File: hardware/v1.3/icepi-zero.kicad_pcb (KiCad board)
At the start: 4 copper layers, 65 x 30 mm, 162 parts, among them J1 Conn_02x20_Counter_Clockwise, J2 GPDI_C_1.3, J3 USB_C_Receptacle_USB2.0_14P, J4 USB_C_Receptacle_USB2.0_14P, J5 USB_C_Receptacle_USB2.0_14P, J6 Micro_SD_Card_Det2, SW1 SW_Push, SW2 SW_Push, U1 ECP5-CABGA256, U10 W9825G6KH, U11 W25Q128JVS, U2 TLV62569DBV, U3 TLV62569DBV, U4 TLV62569DBV, U5 PCA9306DC1, U6 FT231XQ, U7 TPD2EUSB30A, U8 TPD2EUSB30A, U9 TPD2EUSB30A, Y1 SG-8018CG 50.000000MHz

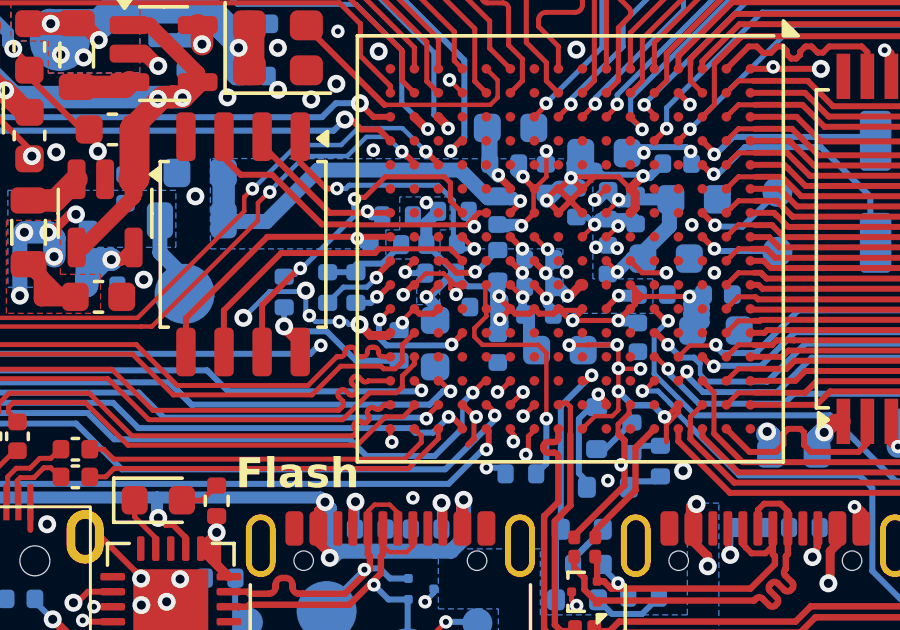
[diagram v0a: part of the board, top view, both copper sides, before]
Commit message: DVI multires
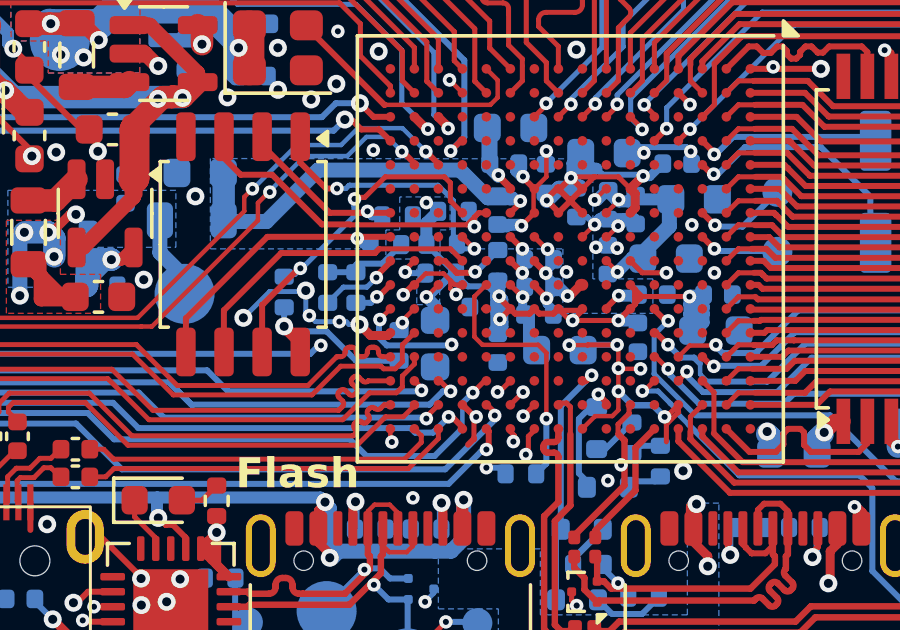
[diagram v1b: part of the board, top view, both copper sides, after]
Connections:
- U1 pad M11: /USB/JTAG_TDO -> unconnected-(U1E-PR47A/+/HS/RSQ44-PadM11)
- U1 pad N12: /USB/JTAG_TMS -> unconnected-(U1E-PR44D/-/RSQ44-PadN12)
- U1 pad P11: /USB/JTAG_TDI -> unconnected-(U1E-PR47C/+/RSQ44/LRC_GPLL0T_IN-PadP11)
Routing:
- net /USB/JTAG_TDI: track 32.6 -> 31.7 mm
- net /USB/JTAG_TMS: track 34.5 -> 34.0 mm
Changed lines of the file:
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@@
 	(net 259 "/GPIO27")
 	(net 260 "unconnected-(U1J-PB18A{slash}WRITEN-PadM9)")
+	(net 261 "unconnected-(U1E-PR44D{slash}-{slash}RSQ44-PadN12)")
+	(net 262 "unconnected-(U1E-PR47C{slash}+{slash}RSQ44{slash}LRC_GPLL0T_IN-PadP11)")
+	(net 263 "unconnected-(U1E-PR47A{slash}+{slash}HS{slash}RSQ44-PadM11)")
 	(footprint "MountingHole:MountingHole_2.7mm_M2.5"
 		(layer "F.Cu")
@@
 			(property pad_prop_bga)
 			(layers "F.Cu" "F.Mask" "F.Paste")
-			(net 5 "/USB/JTAG_TDO")
+			(net 263 "unconnected-(U1E-PR47A{slash}+{slash}HS{slash}RSQ44-PadM11)")
 			(pinfunction "PR47A/+/HS/RSQ44")
 			(pintype "bidirectional")
@@
 			(property pad_prop_bga)
 			(layers "F.Cu" "F.Mask" "F.Paste")
-			(net 8 "/USB/JTAG_TMS")
+			(net 261 "unconnected-(U1E-PR44D{slash}-{slash}RSQ44-PadN12)")
 			(pinfunction "PR44D/-/RSQ44")
 			(pintype "bidirectional")
@@
 			(property pad_prop_bga)
 			(layers "F.Cu" "F.Mask" "F.Paste")
-			(net 4 "/USB/JTAG_TDI")
+			(net 262 "unconnected-(U1E-PR47C{slash}+{slash}RSQ44{slash}LRC_GPLL0T_IN-PadP11)")
 			(pinfunction "PR47C/+/RSQ44/LRC_GPLL0T_IN")
 			(pintype "bidirectional")
@@
 		(net 4)
 	)
-	(segment
-		(start 144.96 106.91)
-		(end 144.8 106.75)
-		(width 0.2)
-		(layer "F.Cu")
-		(net 4)
-	)
-	(segment
-		(start 145.44 106.91)
-		(end 144.96 106.91)
-		(width 0.2)
-		(layer "F.Cu")
-		(net 4)
-	)
-	(segment
-		(start 145.6 106.75)
-		(end 145.44 106.91)
-		(width 0.2)
-		(layer "F.Cu")
-		(net 4)
-	)
 	(via
 		(at 144.399998 107.209961)
@@
 	)
 	(segment
-		(start 148.931745 107.95)
-		(end 149.199998 108.218253)
+		(start 147.19 105.95)
+		(end 146.8 106.34)
 		(width 0.15)
 		(layer "F.Cu")
@@
 	)
 	(segment
-		(start 149.199998 108.218253)
-		(end 149.199999 110.40996)
+		(start 148.931745 107.95)
+		(end 149.199998 108.218253)
 		(width 0.15)
 		(layer "F.Cu")
@@
 	)
 	(segment
-		(start 146.8 107.681745)
-		(end 147.068255 107.95)
+		(start 146.8 106.34)
+		(end 146.8 107.681745)
 		(width 0.15)
 		(layer "F.Cu")
@@
 	)
 	(segment
-		(start 145.85 117.185)
-		(end 145.355 117.68)
-		(width 0.17)
-		(layer "F.Cu")
-		(net 5)
-	)
-	(segment
-		(start 147.2 107)
-		(end 146.8 107.4)
+		(start 146.8 107.681745)
+		(end 147.068255 107.95)
 		(width 0.15)
 		(layer "F.Cu")
@@
 	)
 	(segment
-		(start 146.8 107.4)
-		(end 146.8 107.681745)
-		(width 0.15)
+		(start 145.85 117.185)
+		(end 145.355 117.68)
+		(width 0.17)
 		(layer "F.Cu")
 		(net 5)
@@
 	)
 	(segment
-		(start 147.2 106.75)
-		(end 147.2 107)
+		(start 147.2 105.95)
+		(end 147.19 105.95)
 		(width 0.15)
 		(layer "F.Cu")
@@
 	)
 	(segment
-		(start 147.165 105.985)
-		(end 147.165 106.715)
+		(start 149.199998 108.218253)
+		(end 149.199999 110.40996)
 		(width 0.15)
 		(layer "F.Cu")
@@
 		(net 8)
 	)
-	(segment
-		(start 146.4 107.580151)
-		(end 146.044151 107.936)
-		(width 0.2)
-		(layer "F.Cu")
-		(net 8)
-	)
 	(via
 		(at 146.044151 107.936)
@@
 		(net 259)
 	)
+	(segment
+		(start 147.2 106.75)
+		(end 147.09 106.75)
+		(width 0.15)
+		(layer "F.Cu")
+		(net 263)
+	)
 	(zone
